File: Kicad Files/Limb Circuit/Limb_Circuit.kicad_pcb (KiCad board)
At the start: 2 copper layers, 84.5 x 49.5 mm, 16 parts, among them J1 XT60_F_16.6V, J2 XT60_F_Heater, J3 XT60_F_Thermocouple, Q1 BUK9M52-40EX, U1 MAX31855KASA+T, U2 LSM6DSL

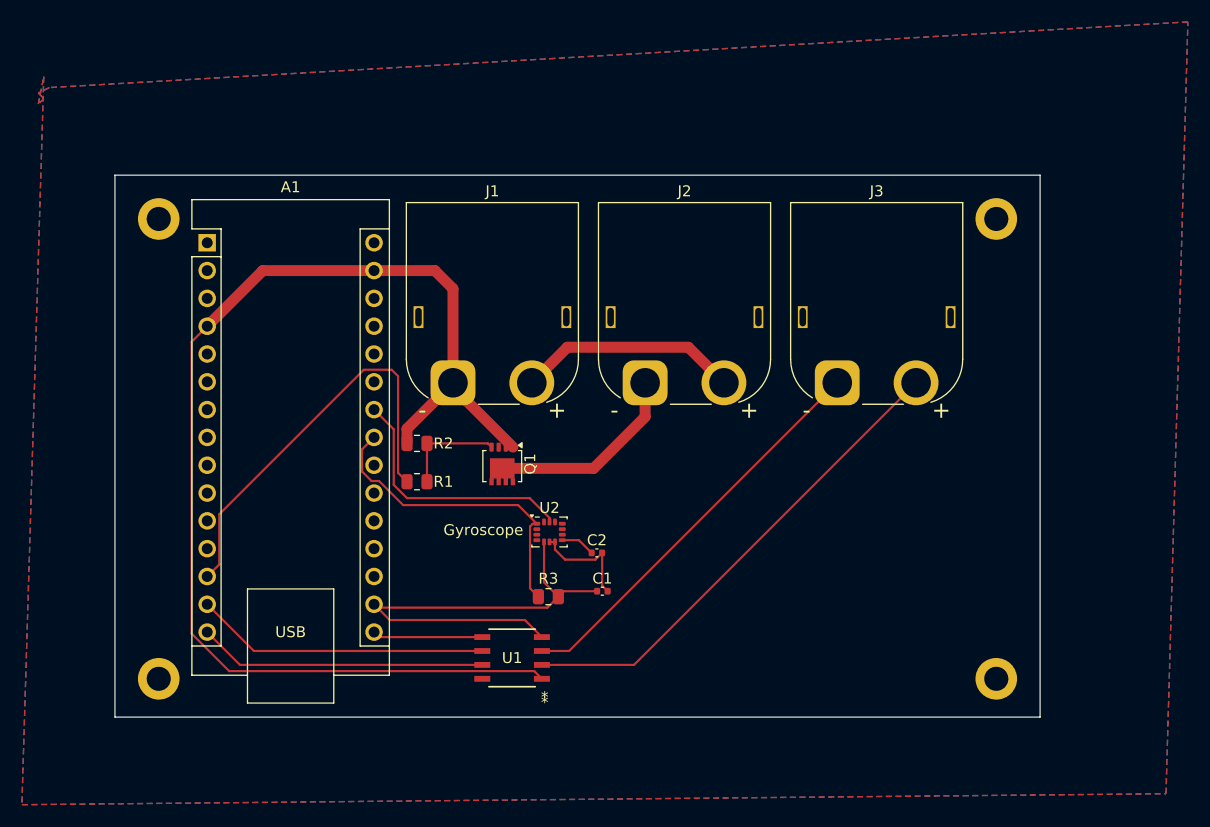
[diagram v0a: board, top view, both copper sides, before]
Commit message: Finished limb circuit board
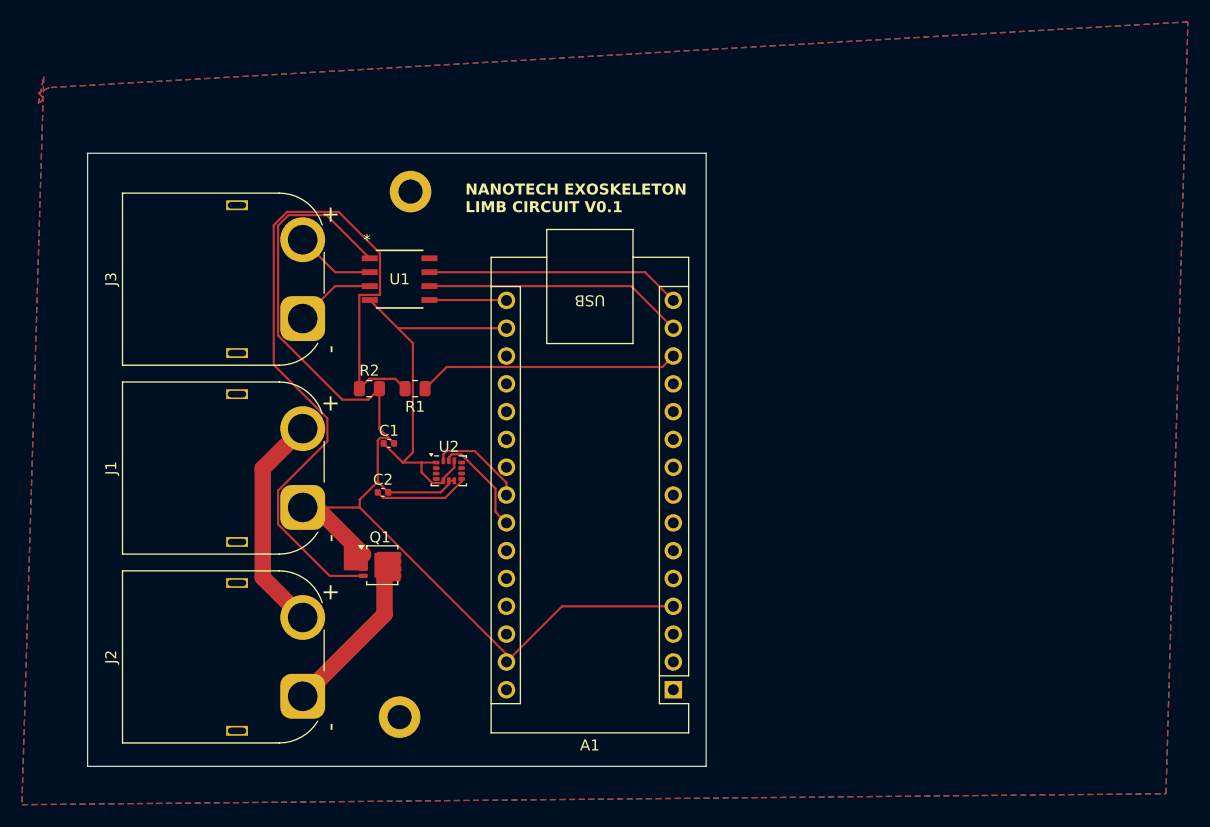
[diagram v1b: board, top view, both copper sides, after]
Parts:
- removed R3: 10k, Resistor_SMD:R_0805_2012Metric
- removed the REF** at (170.0, 151.5)
- removed the REF** at (170.0, 109.5)
- removed the REF** at (93.5, 109.5)
- removed the REF** at (93.5, 151.5)
- added REF**: MountingHole_2.2mm_M2_DIN965_Pad, MountingHole:MountingHole_2.2mm_M2_DIN965_Pad, F.Cu at (115.5, 155.0)
- added REF**: MountingHole_2.2mm_M2_DIN965_Pad, MountingHole:MountingHole_2.2mm_M2_DIN965_Pad, F.Cu at (116.5, 107.0)
- moved A1 59.0 mm to (140.5, 152.5), turned to 180 degrees
- moved J3 49.2 mm to (106.7, 118.6), turned to 90 degrees
- moved J2 42.4 mm to (106.7, 153.1), turned to 90 degrees
- moved U1 36.1 mm to (115.5, 115.0), turned to 0 degrees
- moved C1 23.7 mm to (114.5, 130.0)
- moved C2 20.3 mm to (114.0, 134.5)
- moved J1 17.8 mm to (106.7, 135.8), turned to 90 degrees
- moved Q1 14.5 mm to (113.7, 141.1), turned to 0 degrees
- moved U2 10.8 mm to (120.0, 132.5)
- moved R1 8.50 mm to (116.9, 125.0), turned to 180 degrees
- moved R2 6.63 mm to (112.7, 125.0), turned to 0 degrees
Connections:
- U2 pad 1: SDA_gyro -> 3.3V_ard
- U2 pad 12: CS_gyro -> 3.3V_ard
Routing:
- net Net-(Q1-G): track 9.54 -> 71.9 mm
- net Net-(J3-Pin_2): track 44.8 -> 7.35 mm
- net Net-(J3-Pin_1): track 37.1 -> 7.35 mm
- net SDA_gyro: track 29.0 -> 8.80 mm
- net GND_16.4V: track 121.5 -> 104.2 mm
- net PWM_heater: track 38.2 -> 23.9 mm
- net SCL_gyro: track 23.5 -> 9.53 mm
- net Net-(U2-VDD): track 3.17 -> 8.72 mm
- net 3.3V_ard: track 43.2 -> 37.9 mm
- net GND_heater: track 18.1 -> 15.1 mm
- net CS_thermocouple: track 26.9 -> 23.9 mm
- net CLK: track 10.1 -> 7.05 mm
- net MISO_thermocouple: track 26.4 -> 23.3 mm
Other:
- board size 84.5 x 49.5 mm -> 56.5 x 56 mm
- board text added: "NANOTECH EXOSKELETON LIMB CIRCUIT V0.1"
- board text removed: "Gyroscope"
